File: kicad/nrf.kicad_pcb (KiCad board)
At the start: 2 copper layers, 17.8 x 38.1 mm, 6 parts, among them P1 ICSP, P2 CONN_01X02, P3 NRF_24L01, U1 MCP1755ST-3302E/DB

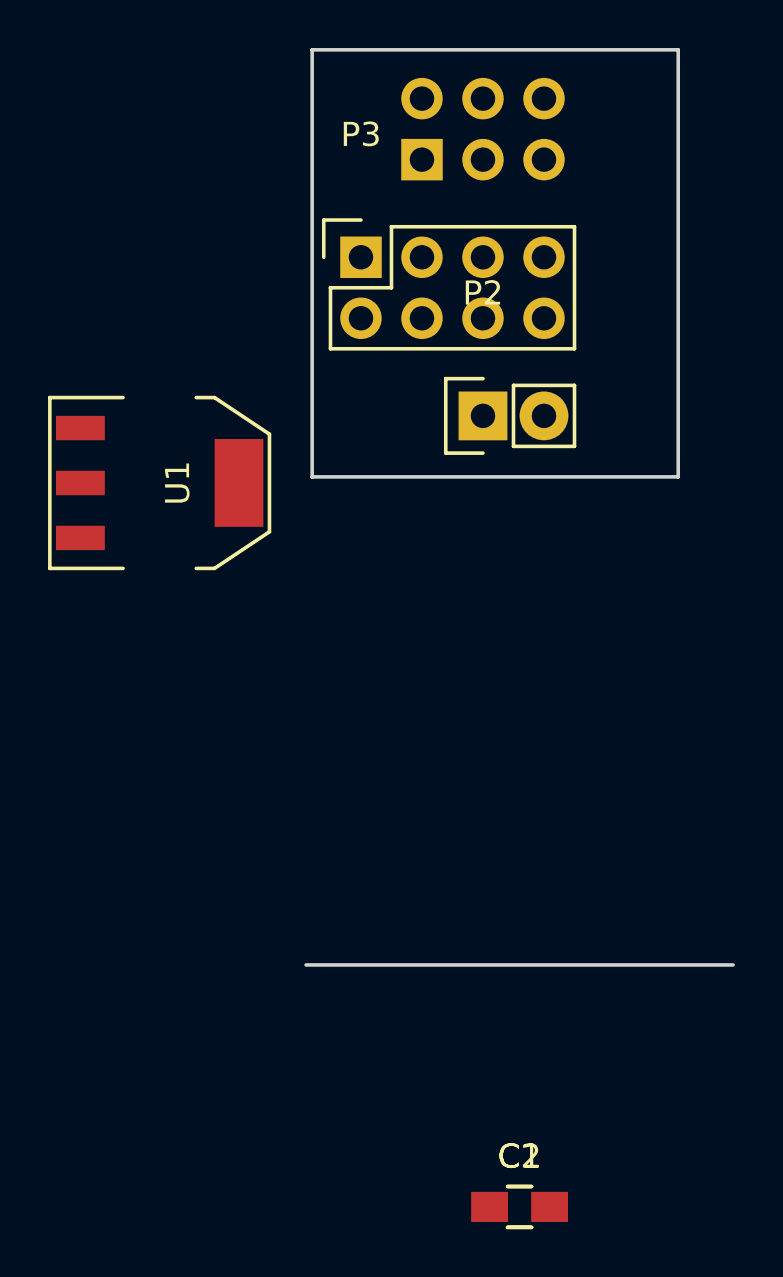
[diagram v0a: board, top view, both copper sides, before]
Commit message: Voltage regulator
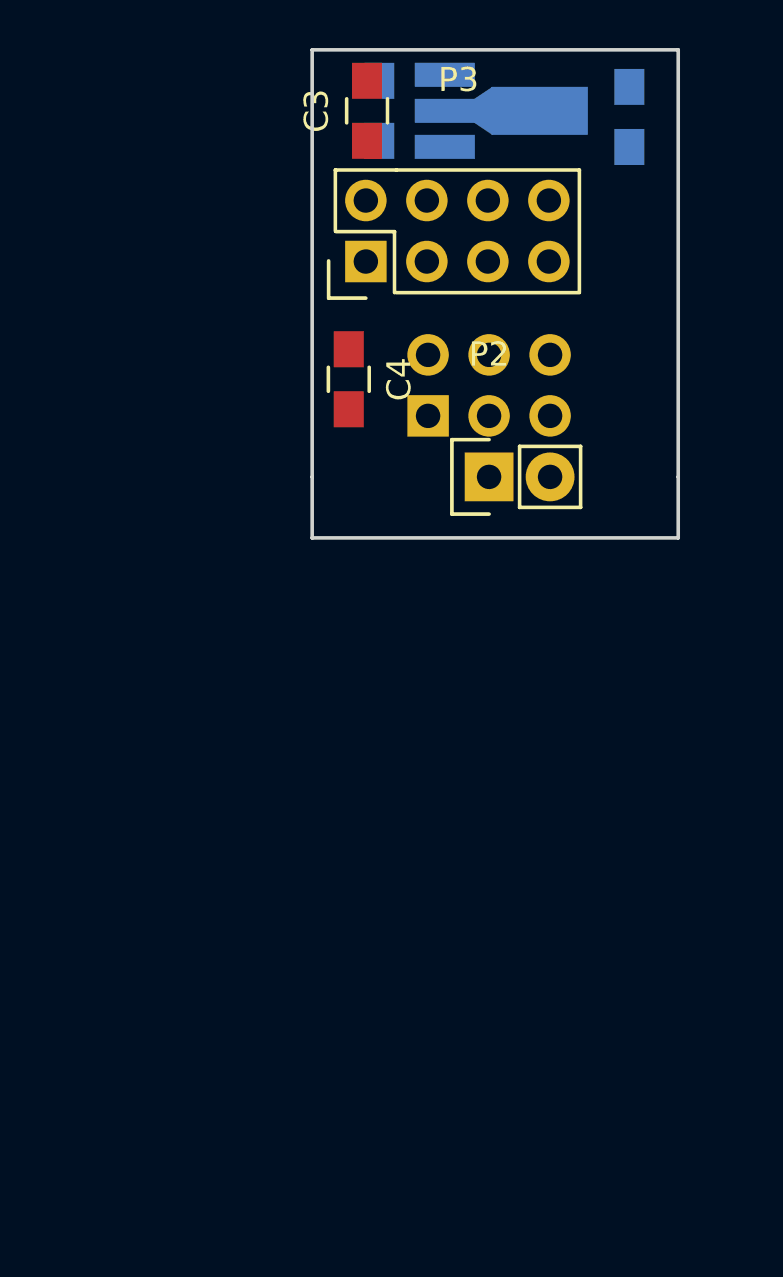
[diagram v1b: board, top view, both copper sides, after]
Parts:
- added C3: 10uF, Capacitors_SMD:C_0805_HandSoldering, F.Cu at (158.7, 89.8)
- added C4: 10uF, Capacitors_SMD:C_0805_HandSoldering, F.Cu at (157.9, 100.9)
- C1, C2: moved to B.Cu
- P3: footprint Socket_Strips:Socket_Strip_Straight_2x04 -> NRF_24L01
- U1: value MCP1755ST-3302E/DB -> MCP1700_SOT-89; footprint TO_SOT_Packages_SMD:SOT-223 -> TO_SOT_Packages_SMD:SOT89-3_Housing_Handsoldering; moved to B.Cu
- moved C2 46.0 mm to (159.2, 89.8), turned to 270 degrees
- moved C1 45.6 mm to (169.6, 90.0), turned to 90 degrees
- moved U1 21.0 mm to (164.2, 89.8), turned to 90 degrees
- moved P1 10.7 mm to (161.2, 102.5)
- moved P3 4.66 mm to (162.5, 93.6)
- moved P2 2.55 mm to (163.7, 105.0)
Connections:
- U1 pad 1: 5V -> GND
- U1 pad 2: GND -> 5V
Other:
- board size 17.8 x 38.1 mm -> 15.2 x 20.3 mm
